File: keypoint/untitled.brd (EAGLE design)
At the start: 88 x 60 mm, 66 parts, among them J3 10103594, K1 351, K2 351, Q1 MMBT3904, Q2 MMBT3904, Q3 12MHz, Q4 S9013, Q5 S9013, U1 AMS1117, U2 MAX232CSE, U3 PC817X2NIP0F, U4 PC817X2NIP0F, U5 MAX232CSE, X1 MSTBA2, X2 MSTBA3

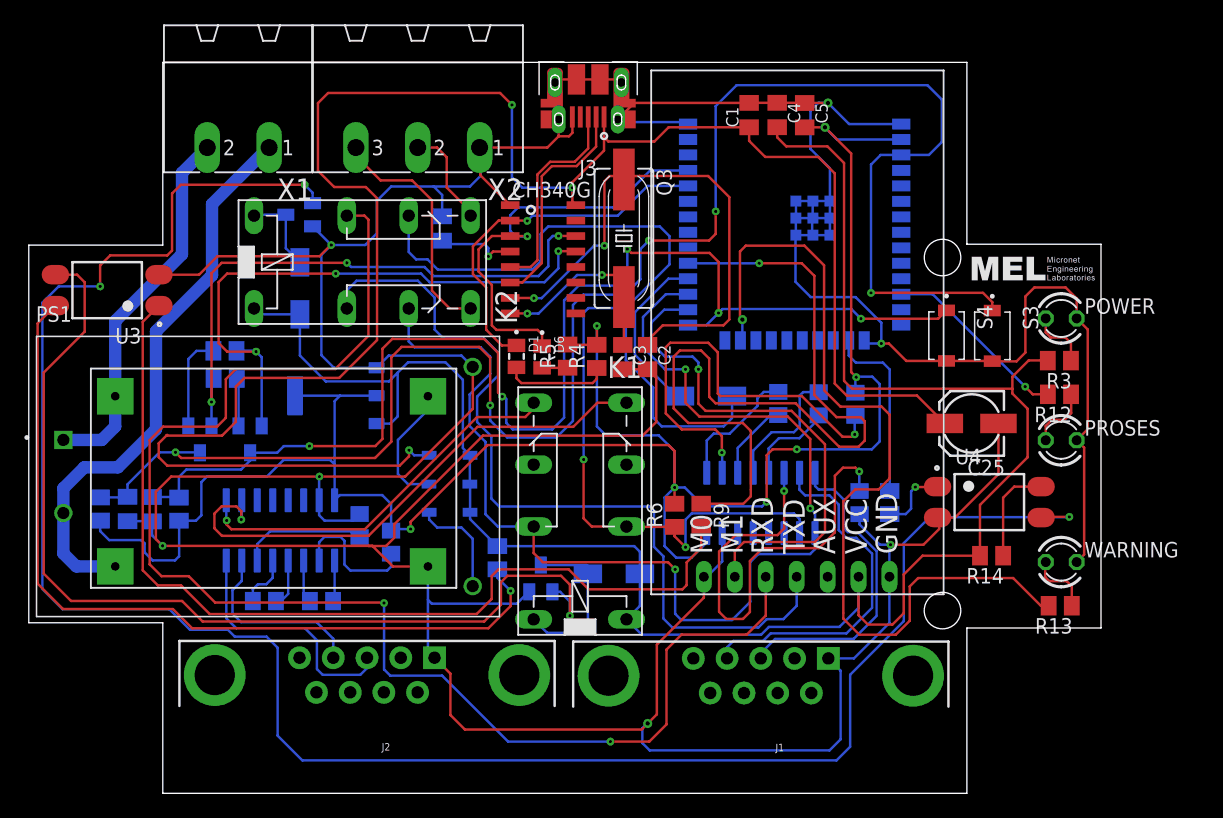
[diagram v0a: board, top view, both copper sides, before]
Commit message: fix PCB versi 1.0
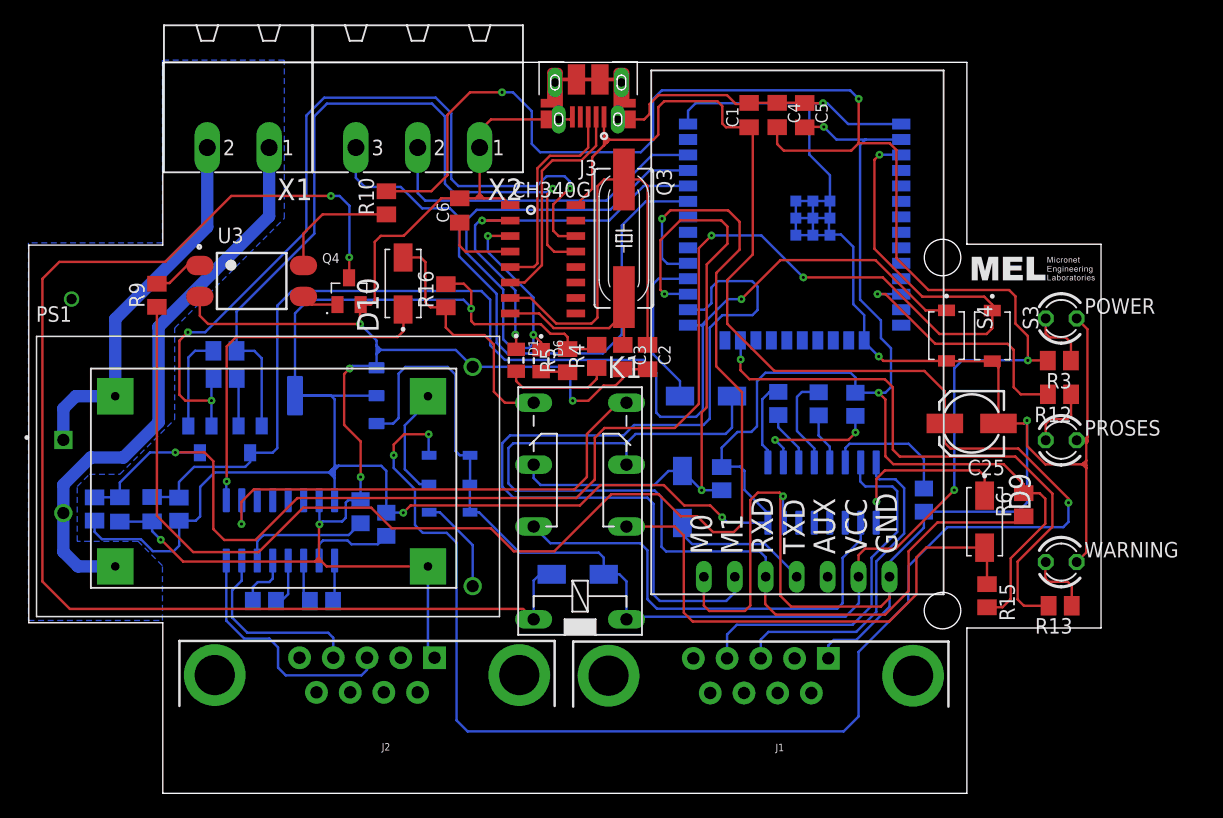
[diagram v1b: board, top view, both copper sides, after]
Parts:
- removed D8: US1M-13, US1M-13:DIOM5226X240N
- removed K2: 351, relay:351
- removed Q5: S9013, S9013:SOT95P240X120-3N
- removed R11: 330, adafruit:M0805
- removed R14: 1k, adafruit:M0805
- removed U4: PC817X2NIP0F, PC817X2NIP0F:SOT254P975X400-4N
- added D10, D11, D9: US1M-13, US1M-13:DIOM5226X240N
- added R15, R16, R17: 10K, adafruit:M0805
- R4, R5: value 1K -> 10K
- moved R9 48.2 mm to (1.55, 42.7), turned to 90 degrees
- moved R10 30.5 mm to (20.4, 50.3), flipped to the top
- moved R6 28.7 mm to (72.7, 25.5)
- moved Q4 28.4 mm to (17.3, 43.0), flipped to the top
- moved U3 11.9 mm to (9.32, 43.9), turned to 0 degrees
- moved C16 5.29 mm to (64.5, 25.9)
- moved U5 5.09 mm to (56.1, 26.5)
- moved D7 2.97 mm to (36.1, 19.8)
- moved C6 2.06 mm to (26.4, 49.7), flipped to the top
- moved C7 1.52 mm to (20.4, 23.9)
- moved C8 1.14 mm to (18.3, 24.9)
- moved C14 0.64 mm to (-1.50, 25.1)
- moved R7 0.46 mm to (-3.57, 25.2)
- moved R5 0.37 mm to (35.3, 37.3)
- moved D1 0.32 mm to (31.0, 37.4)
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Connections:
- removed net N$30: R11.2, U4.1
- removed net N$31: R14.1, U4.4
- removed net N$33: D8.A, K2.16, Q5.3
- removed net N$36: Q5.1, U4.3
- removed net RXLORA_CONFIG: K2.S2, X2.2
- removed net TXLORA_CONFIG: K2.S1, X2.3
- new net N$38: D9.C, U5.9
- new net N$39: D10.C, U2.9
- new net N$40: D11.C, EBYTEE220-900T22D1.TXD
- new net SCL: MD1.36, X2.2
- new net SDA: MD1.33, X2.3
- net 3V3: now also R15.2, R16.2, R17.2
- net GND: no longer Q5.2, U4.2
- net OUT+: no longer D8.C, K2.1, R14.2
- net RXLORA: now also D5.A, K1.O1, R6.1; no longer K2.P2
- net RX_DB9: now also D9.A, K1.P1, R15.1; no longer K1.P2, K2.O1, MD1.27, U5.9
- net RX_DB9-1: now also D10.A, R16.1; no longer U2.9
- net SW_LORACONFIG: no longer R11.1
- net TXLORA: now also D11.A, K1.O2, MD1.27, R17.1; no longer EBYTEE220-900T22D1.TXD, K2.P1
- net TX_DB9: now also K1.P2; no longer D5.A, K1.P1, K2.O2, R6.1
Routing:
- net N$36: track 166.8 -> 0.00 mm, vias 3 -> 0
- net N$29: track 14.0 -> 105.6 mm, vias 0 -> 2
- net GND: track 430.6 -> 351.4 mm, vias 7 -> 10
- net N$18: track 81.2 -> 3.07 mm, vias 1 -> 0
- net N$15: track 77.1 -> 4.18 mm
- net TX_DB9: track 97.7 -> 37.9 mm, vias 2 -> 0
- net N$16: track 68.0 -> 10.1 mm, vias 1 -> 0
- net RX_DB9: track 97.1 -> 43.7 mm, vias 3 -> 0
- net SDA: track 0.00 -> 50.4 mm
- net 3V3: track 175.3 -> 218.2 mm, vias 7 -> 5
- net SW_MODEM: track 69.4 -> 112.0 mm
- net RXLORA: track 115.9 -> 83.1 mm, vias 2 -> 0
- net M1: track 42.2 -> 71.9 mm, vias 1 -> 0
- net N$39: track 0.00 -> 29.5 mm, vias 0 -> 1
- net N$27: track 39.5 -> 10.7 mm, vias 2 -> 0
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- added copper zone on layer 16, net GROUNDING
